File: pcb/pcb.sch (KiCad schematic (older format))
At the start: 48 parts

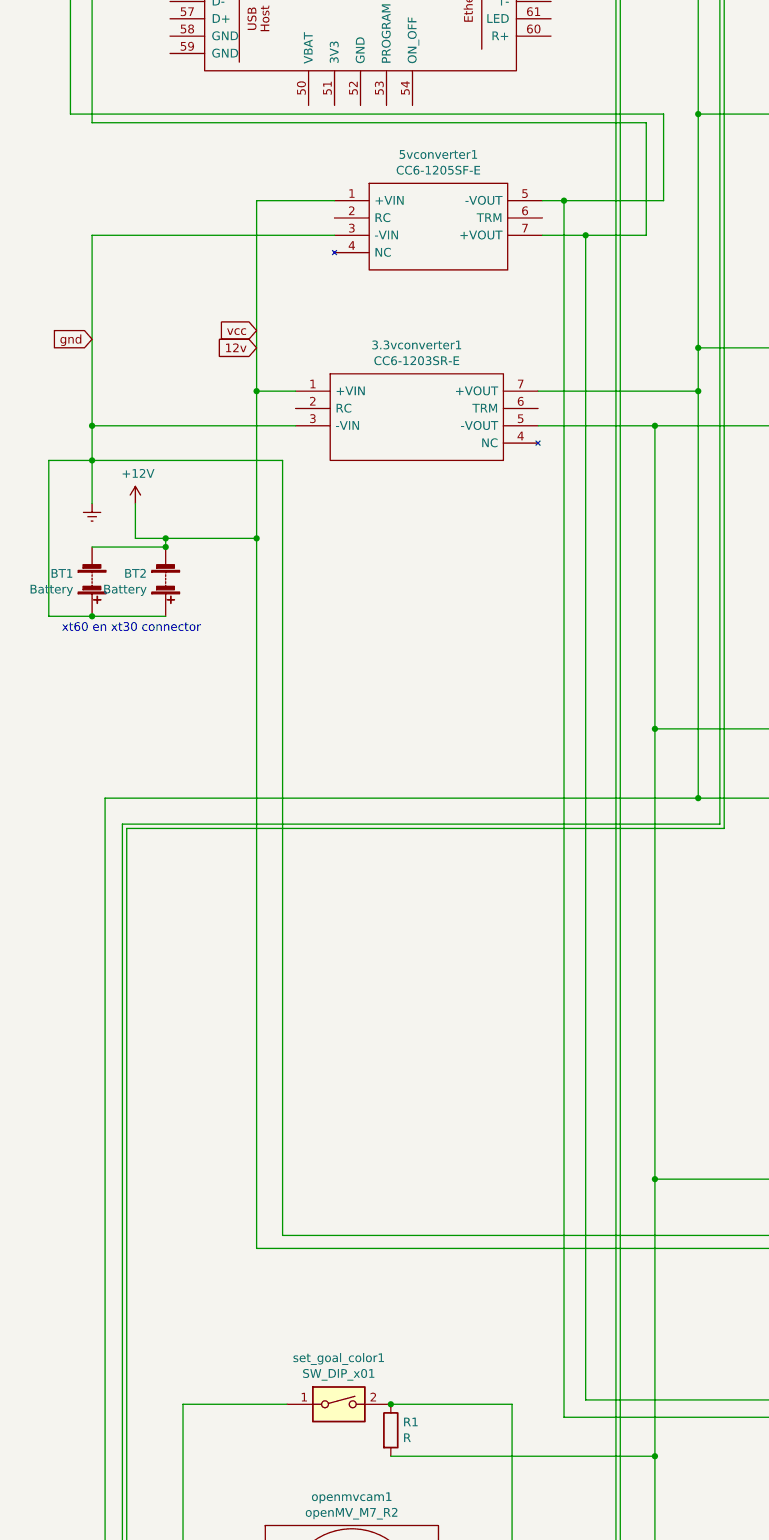
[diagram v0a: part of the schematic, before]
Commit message: Commit message
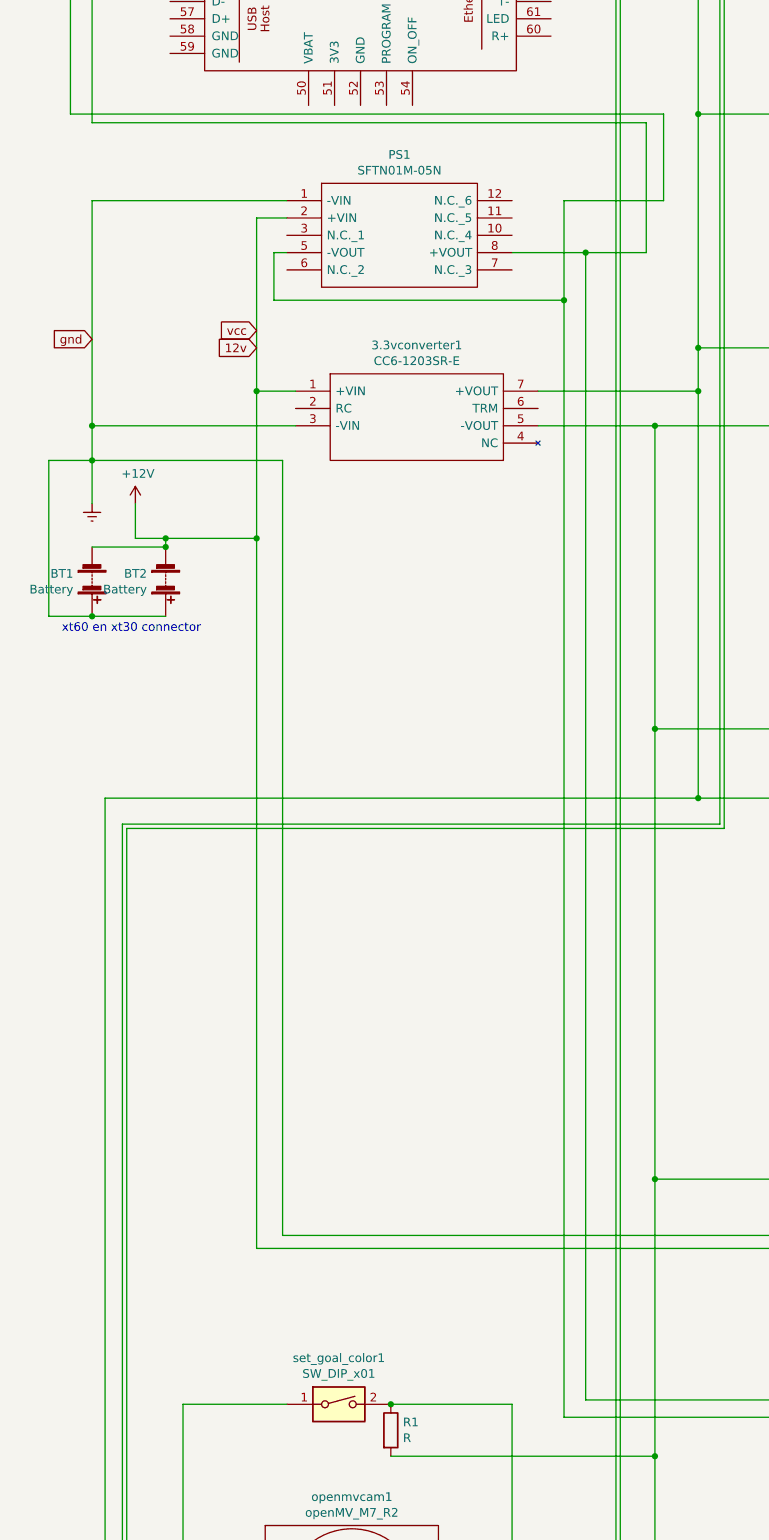
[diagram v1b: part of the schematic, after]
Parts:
- removed 5vconverter1: CC6-1205SF-E, CC6_SF, symbol cc6-1205sf-e:CC6-1205SF-E
- added PS1: SFTN01M-05N, custom:SFTN01M05N, symbol sftn01m-05n:SFTN01M-05N
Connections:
- net +12V: now also PS1.2 (+VIN)
- net Earth: now also PS1.1 (-VIN)
- net at BZ1.2 (+), Motor_driver2.6 (gnd), R2.2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: now also PS1.5 (-VOUT)
- net at Motor_driver2.7 (vcc), controllboard1.48 (VIN), kompas1.3 (vin(2.5-5v))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: now also PS1.8 (+VOUT)
- net at motor_driver1.12 (pwm): now also io_expender2.6 (GPB5)
- net at Motor_driver2.12 (pwm): now also io_expender2.2 (GPB1)
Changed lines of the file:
@@
 $EndComp
-Wire Wire Line
-	1800 5400 1800 6500
 Wire Wire Line
 	3425 6500 4350 6500
@@
 Wire Wire Line
 	1800 6500 2025 6500
-Connection ~ 1800 6500
 Wire Wire Line
 	1800 6500 1800 7350
@@
 Wire Wire Line
 	850  6700 850  6900
-$Comp
-L cc6-1205sf-e:CC6-1205SF-E 5vconverter1
-U 1 1 66A897F1
-P 2250 5400
-F 0 "5vconverter1" H 2850 5665 50  0000 C CNN
-F 1 "CC6-1205SF-E" H 2850 5574 50  0000 C CNN
-F 2 "CC6_SF" H 3300 5500 50  0001 L CNN
-F 3 "https://product.tdk.com/system/files/dam/doc/product/power/switching-power/dc-dc-converter/catalog/cc-e_e.pdf" H 3300 5400 50  0001 L CNN
-F 4 "dcdc,convertor TDK-Lambda Through Hole Isolated DC-DC Converter, I/O isolation 500V ac, Vout 5V dc" H 3300 5300 50  0001 L CNN "Description"
-F 5 "TDK" H 3300 5100 50  0001 L CNN "Manufacturer_Name"
-F 6 "CC6-1205SF-E" H 3300 5000 50  0001 L CNN "Manufacturer_Part_Number"
-F 7 "967-CC6-1205SF-E" H 3300 4900 50  0001 L CNN "Mouser Part Number"
-F 8 "https://www.mouser.co.uk/ProductDetail/TDK-Lambda/CC6-1205SF-E?qs=Vwh6e7toGLhaPHzXVKmH%252BA%3D%3D" H 3300 4800 50  0001 L CNN "Mouser Price/Stock"
-F 9 "CC6-1205SF-E" H 3300 4700 50  0001 L CNN "Arrow Part Number"
-F 10 "https://www.arrow.com/en/products/cc6-1205sf-e/tdk-lambda-americas?region=nac" H 3300 4600 50  0001 L CNN "Arrow Price/Stock"
-	1    2250 5400
-	1    0    0    -1
-$EndComp
-Wire Wire Line
-	2250 5400 1800 5400
-Wire Wire Line
-	2250 5600 850  5600
-Wire Wire Line
-	850  5600 850  6700
-Wire Wire Line
-	3450 5400 3575 5400
 Wire Wire Line
 	4150 5400 4150 4900
 Wire Wire Line
-	3575 5400 3575 12425
-Connection ~ 3575 5400
-Wire Wire Line
 	3575 5400 4150 5400
 Wire Wire Line
-	3450 5600 3700 5600
-Wire Wire Line
-	4050 5600 4050 4950
-Wire Wire Line
-	3700 12325 3700 5600
-Connection ~ 3700 5600
-Wire Wire Line
-	3700 5600 4050 5600
+	3700 12325 3700 5700
 $Comp
 L tb9051ftg:TB9051FTG motor_driver1
@@
 Connection ~ 19100 7900
 Connection ~ 20475 12425
+$Comp
+L sftn01m-05n:SFTN01M-05N PS1
+U 1 1 66490BE8
+P 1975 5400
+F 0 "PS1" H 2625 5665 50  0000 C CNN
+F 1 "SFTN01M-05N" H 2625 5574 50  0000 C CNN
+F 2 "custom:SFTN01M05N" H 3125 5500 50  0001 L CNN
+F 3 "https://www.meanwell.com/webapp/product/search.aspx?prod=SFTN01-N" H 3125 5400 50  0001 L CNN
+F 4 "Isolated DC/DC Converters - SMD 1W 12Vin 5Vout 20-200mA SMT Unregulated" H 3125 5300 50  0001 L CNN "Description"
+F 5 "7.6" H 3125 5200 50  0001 L CNN "Height"
+F 6 "Mean Well" H 3125 5100 50  0001 L CNN "Manufacturer_Name"
+F 7 "SFTN01M-05N" H 3125 5000 50  0001 L CNN "Manufacturer_Part_Number"
+F 8 "709-SFTN01M-05N" H 3125 4900 50  0001 L CNN "Mouser Part Number"
+F 9 "https://www.mouser.co.uk/ProductDetail/MEAN-WELL/SFTN01M-05N?qs=A6eO%252BMLsxmQLvWwJN5Fn%252BQ%3D%3D" H 3125 4800 50  0001 L CNN "Mouser Price/Stock"
+	1    1975 5400
+	1    0    0    -1
+$EndComp
+Wire Wire Line
+	1800 6500 1800 5500
+Wire Wire Line
+	1800 5500 1975 5500
+Connection ~ 1800 6500
+Wire Wire Line
+	1975 5400 850  5400
+Wire Wire Line
+	850  5400 850  6700
+Wire Wire Line
+	1975 5700 1900 5700
+Wire Wire Line
+	1900 5700 1900 5975
+Wire Wire Line
+	3275 5700 3700 5700
+Connection ~ 3700 5700
+Wire Wire Line
+	4050 5700 3700 5700
+Wire Wire Line
+	4050 4950 4050 5700
+Wire Wire Line
+	1900 5975 3575 5975
+Wire Wire Line
+	3575 5400 3575 5975
+Connection ~ 3575 5975
+Wire Wire Line
+	3575 5975 3575 12425
 $EndSCHEMATC

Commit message: pcb onder gemaakt
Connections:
- net at motor_driver1.12 (pwm): now also io_expender2.6 (GPB5)
- net at Motor_driver2.12 (pwm): now also io_expender2.2 (GPB1)
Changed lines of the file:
@@
 Connection ~ 10850 2300
-$Comp
-L Device:R R2
-U 1 1 675AF867
-P 11500 2725
-F 0 "R2" H 11570 2771 50  0000 L CNN
-F 1 "R" H 11570 2680 50  0000 L CNN
-F 2 "custom:resistor" V 11430 2725 50  0001 C CNN
-F 3 "~" H 11500 2725 50  0001 C CNN
-	1    11500 2725
-	1    0    0    -1
-$EndComp
 $Comp
 L Device:R R3
@@
 Wire Wire Line
 	3575 5975 3575 12425
+$Comp
+L Device:R R2
+U 1 1 675AF867
+P 11500 2725
+F 0 "R2" H 11570 2771 50  0000 L CNN
+F 1 "R" H 11570 2680 50  0000 L CNN
+F 2 "custom:resistor" V 11430 2725 50  0001 C CNN
+F 3 "~" H 11500 2725 50  0001 C CNN
+	1    11500 2725
+	1    0    0    -1
+$EndComp
 $EndSCHEMATC
